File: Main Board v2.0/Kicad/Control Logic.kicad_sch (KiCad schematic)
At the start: 24 parts, among them J2 +3V3 Supply, J3 JTAG, U7 XC95288XL-TQ144, U8 AP1117-33

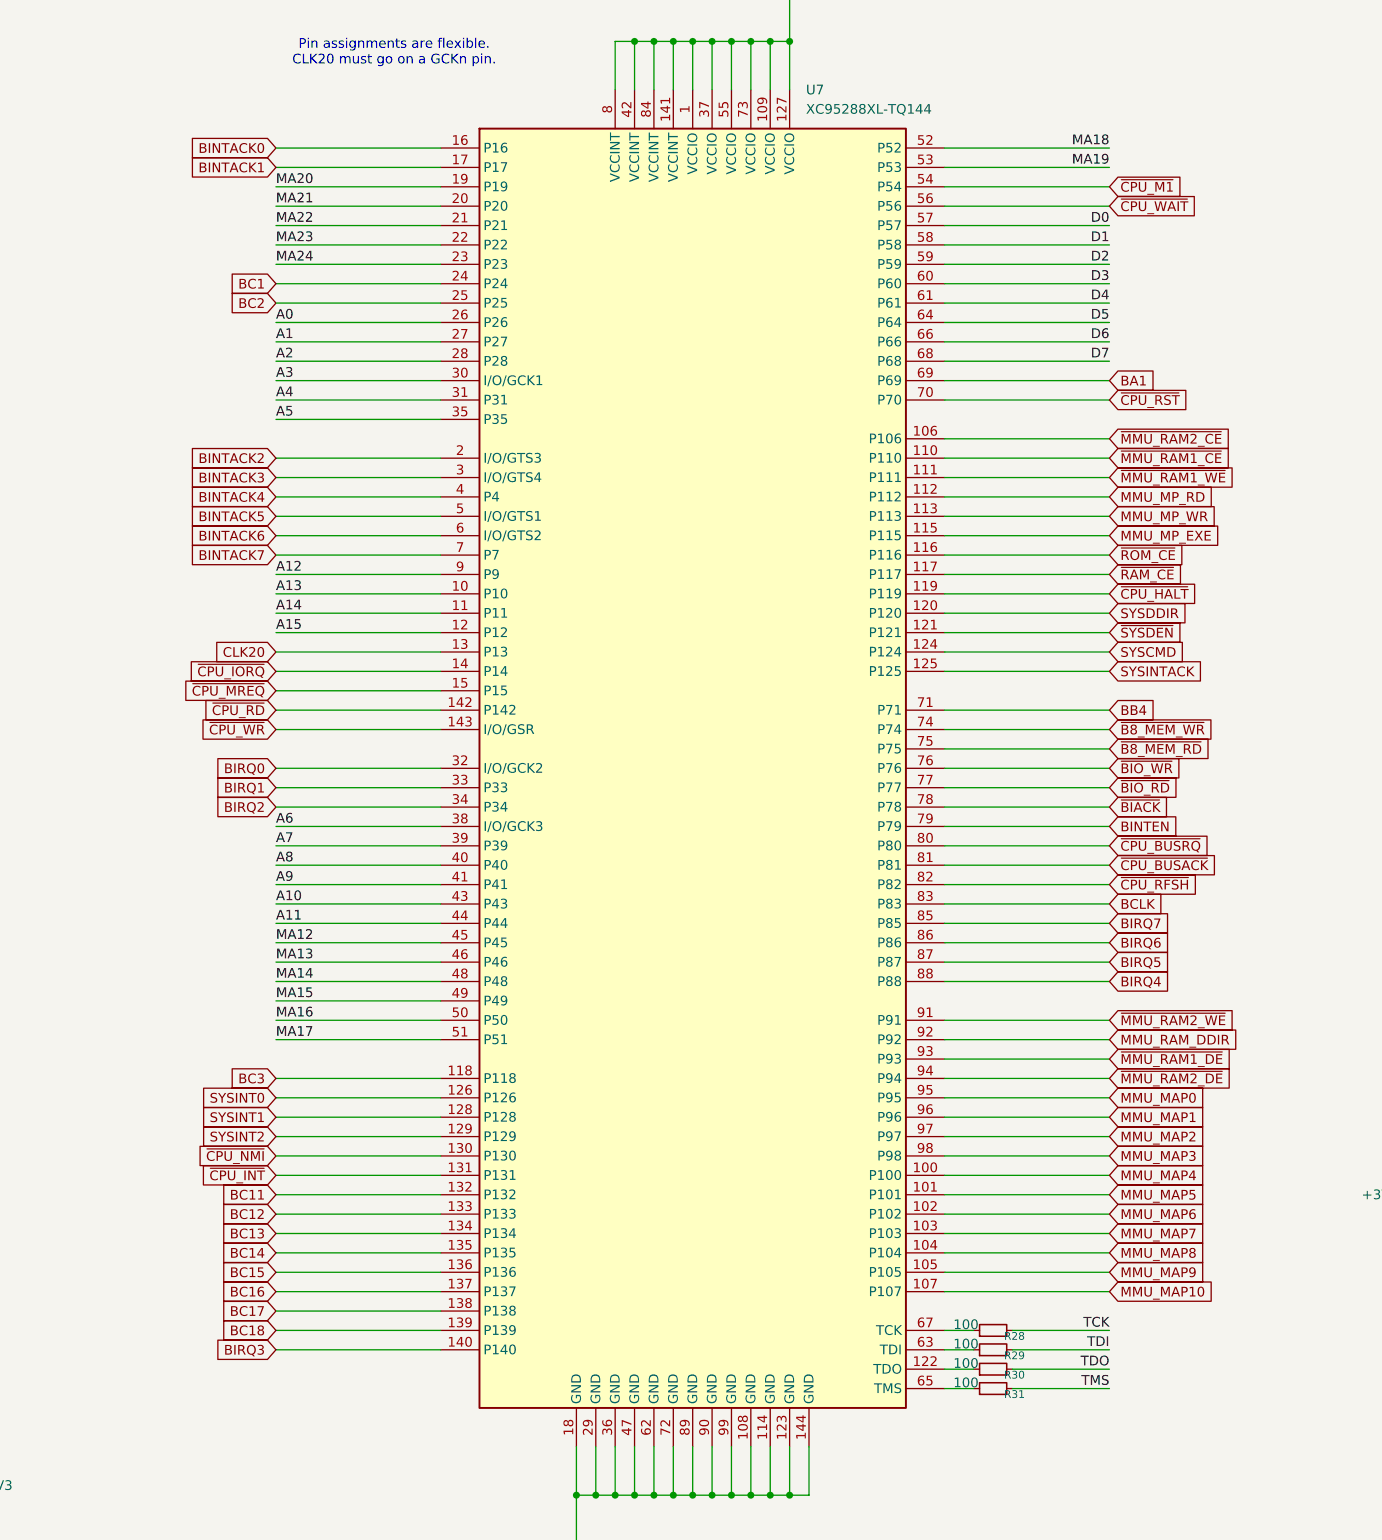
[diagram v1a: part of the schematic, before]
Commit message: board update
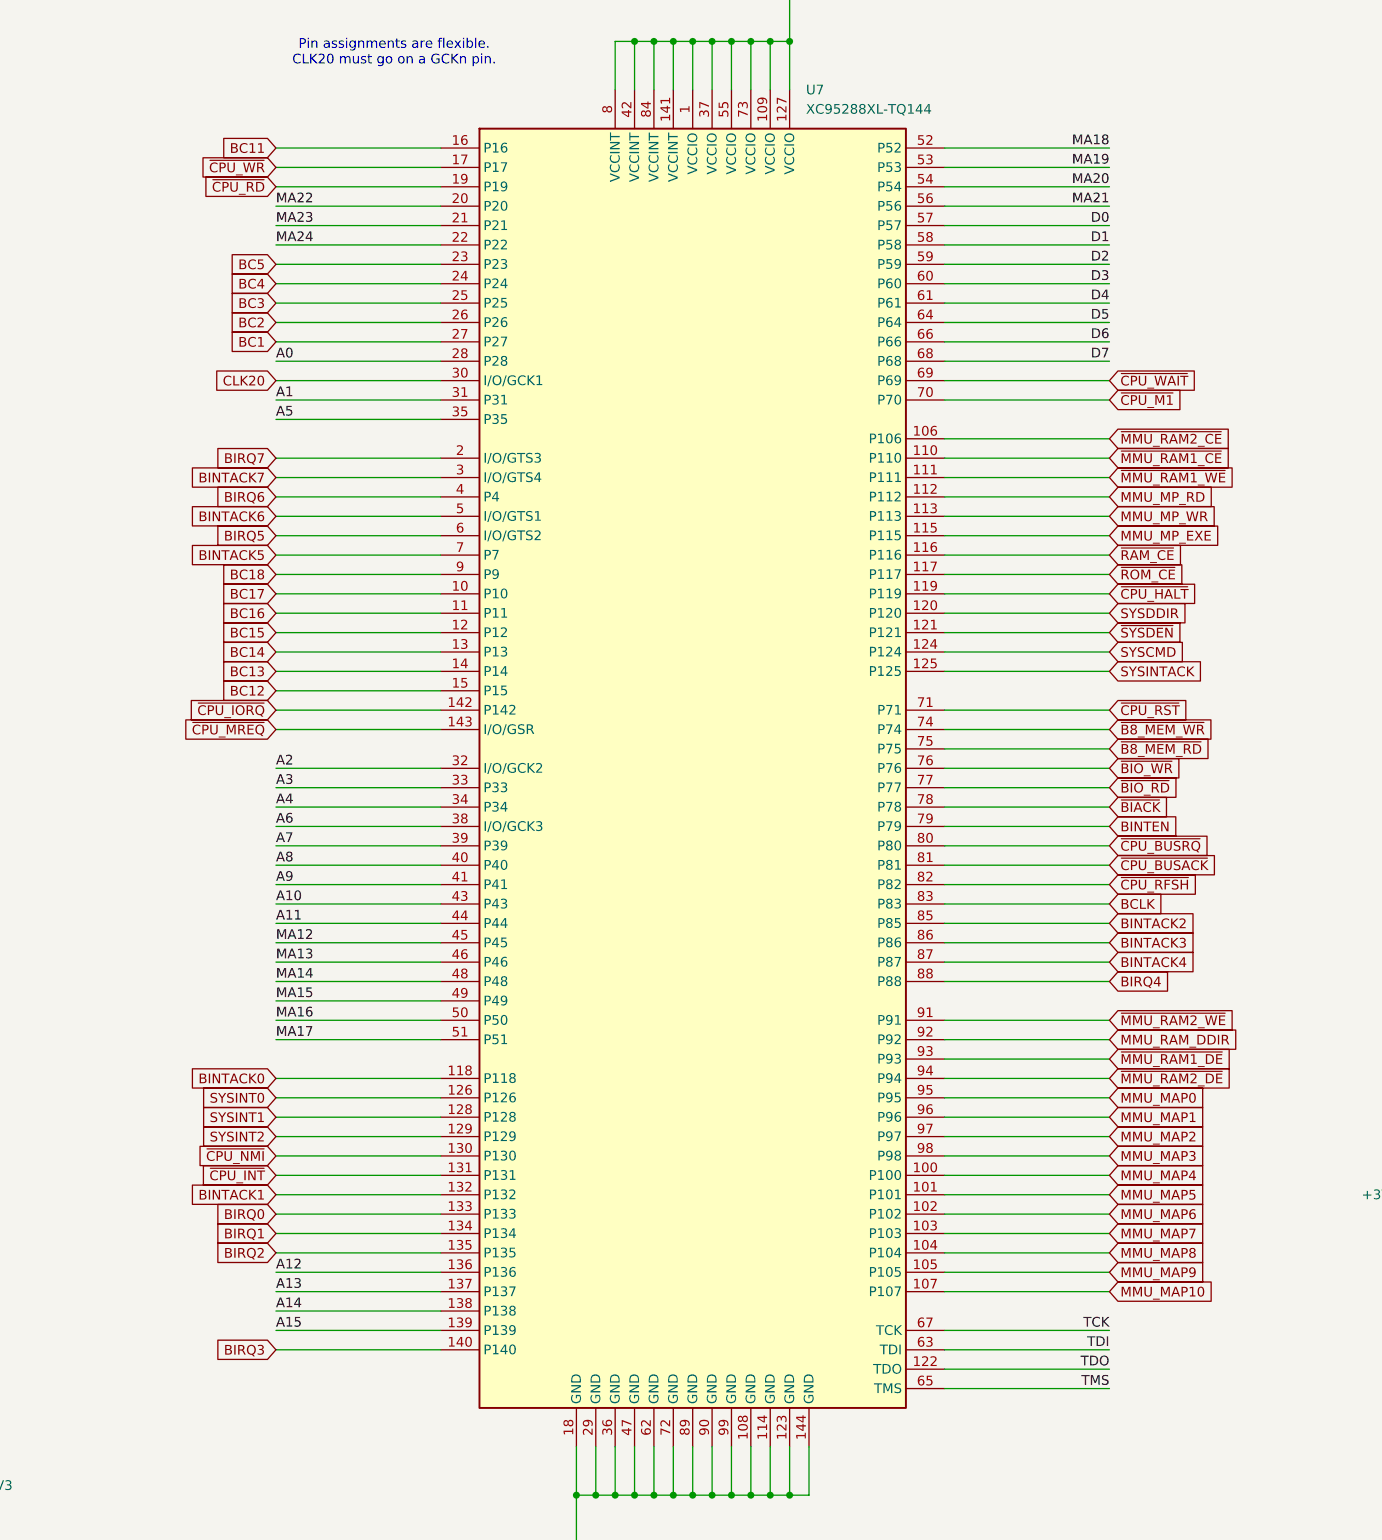
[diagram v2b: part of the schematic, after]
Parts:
- removed R28, R29, R30, R31: 100, Resistor_SMD:R_0603_1608Metric_Pad0.98x0.95mm_HandSolder, symbol Device:R_Small
- C10, C11, C12, C13, C14, C15, C16, C17, C7, C8, C9, R32, R33, R34: KiLib_Generator (none) -> SMD_2terminal_chip_molded
- C18, C19: KiLib_Generator (none) -> capacitor/THT/other
- J2, J3: KiLib_Generator (none) -> connector/pin_header_socket
- U7: KiLib_Generator (none) -> package/gullwing
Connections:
- net BA1 is gone; now on net ~{CPU_WAIT}: U7.69 (P69)
- net BB4 is gone; now on net ~{CPU_RST}: U7.71 (P71)
- net A0: now also U7.28 (P28); no longer U7.26 (P26)
- net A1: now also U7.31 (P31); no longer U7.27 (P27)
- net A12: now also U7.136 (P136); no longer U7.9 (P9)
- net A13: now also U7.137 (P137); no longer U7.10 (P10)
- net A14: now also U7.138 (P138); no longer U7.11 (P11)
- net A15: now also U7.139 (P139); no longer U7.12 (P12)
- net A2: now also U7.32 (I/O/GCK2); no longer U7.28 (P28)
- net A3: now also U7.33 (P33); no longer U7.30 (I/O/GCK1)
- net A4: now also U7.34 (P34); no longer U7.31 (P31)
- net BC1: now also U7.27 (P27); no longer U7.24 (P24)
- net BC11: now also U7.16 (P16); no longer U7.132 (P132)
- net BC12: now also U7.15 (P15); no longer U7.133 (P133)
- net BC13: now also U7.14 (P14); no longer U7.134 (P134)
- net BC14: now also U7.13 (P13); no longer U7.135 (P135)
- net BC15: now also U7.12 (P12); no longer U7.136 (P136)
- net BC16: now also U7.11 (P11); no longer U7.137 (P137)
- net BC17: now also U7.10 (P10); no longer U7.138 (P138)
- net BC18: now also U7.9 (P9); no longer U7.139 (P139)
- net BC2: now also U7.26 (P26); no longer U7.25 (P25)
- net BC3: now also U7.25 (P25); no longer U7.118 (P118)
- net BINTACK0: now also U7.118 (P118); no longer U7.16 (P16)
- net BINTACK1: now also U7.132 (P132); no longer U7.17 (P17)
- net BINTACK2: now also U7.85 (P85); no longer U7.2 (I/O/GTS3)
- net BINTACK3: now also U7.86 (P86); no longer U7.3 (I/O/GTS4)
- net BINTACK4: now also U7.87 (P87); no longer U7.4 (P4)
- net BINTACK5: now also U7.7 (P7); no longer U7.5 (I/O/GTS1)
- net BINTACK6: now also U7.5 (I/O/GTS1); no longer U7.6 (I/O/GTS2)
- net BINTACK7: now also U7.3 (I/O/GTS4); no longer U7.7 (P7)
- net BIRQ0: now also U7.133 (P133); no longer U7.32 (I/O/GCK2)
- net BIRQ1: now also U7.134 (P134); no longer U7.33 (P33)
- net BIRQ2: now also U7.135 (P135); no longer U7.34 (P34)
- net BIRQ5: now also U7.6 (I/O/GTS2); no longer U7.87 (P87)
- net BIRQ6: now also U7.4 (P4); no longer U7.86 (P86)
- net BIRQ7: now also U7.2 (I/O/GTS3); no longer U7.85 (P85)
- net CLK20: now also U7.30 (I/O/GCK1); no longer U7.13 (P13)
- net MA20: now also U7.54 (P54); no longer U7.19 (P19)
- net MA21: now also U7.56 (P56); no longer U7.20 (P20)
- net MA22: now also U7.20 (P20); no longer U7.21 (P21)
- net MA23: now also U7.21 (P21); no longer U7.22 (P22)
- net MA24: now also U7.22 (P22); no longer U7.23 (P23)
- net TCK: now also U7.67 (TCK)
- net TDI: now also U7.63 (TDI)
- net TDO: now also U7.122 (TDO)
- net TMS: now also U7.65 (TMS)
- net ~{CPU_IORQ}: now also U7.142 (P142); no longer U7.14 (P14)
- net ~{CPU_M1}: now also U7.70 (P70); no longer U7.54 (P54)
- net ~{CPU_MREQ}: now also U7.143 (I/O/GSR); no longer U7.15 (P15)
- net ~{CPU_RD}: now also U7.19 (P19); no longer U7.142 (P142)
- net ~{CPU_RST}: no longer U7.70 (P70)
- net ~{CPU_WAIT}: no longer U7.56 (P56)
- net ~{CPU_WR}: now also U7.17 (P17); no longer U7.143 (I/O/GSR)
- net ~{RAM_CE}: now also U7.116 (P116); no longer U7.117 (P117)
- net ~{ROM_CE}: now also U7.117 (P117); no longer U7.116 (P116)
- new net BC4: U7.24 (P24)
- new net BC5: U7.23 (P23)

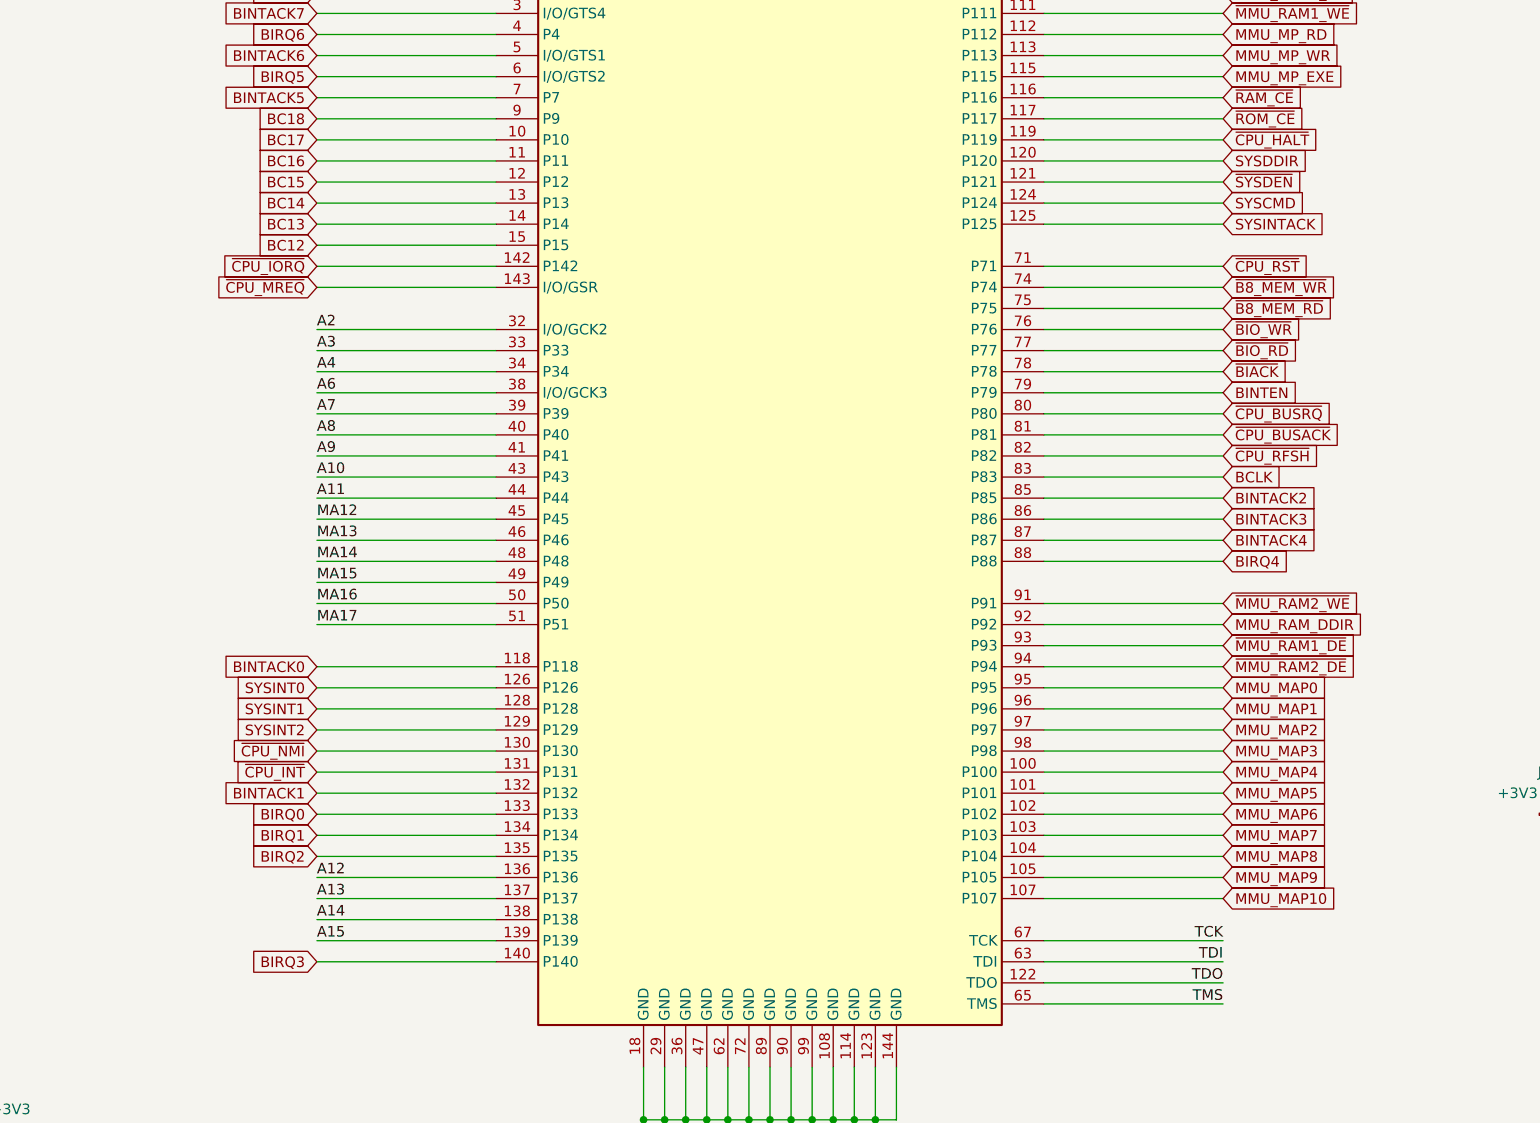
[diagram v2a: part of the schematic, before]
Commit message: board progress
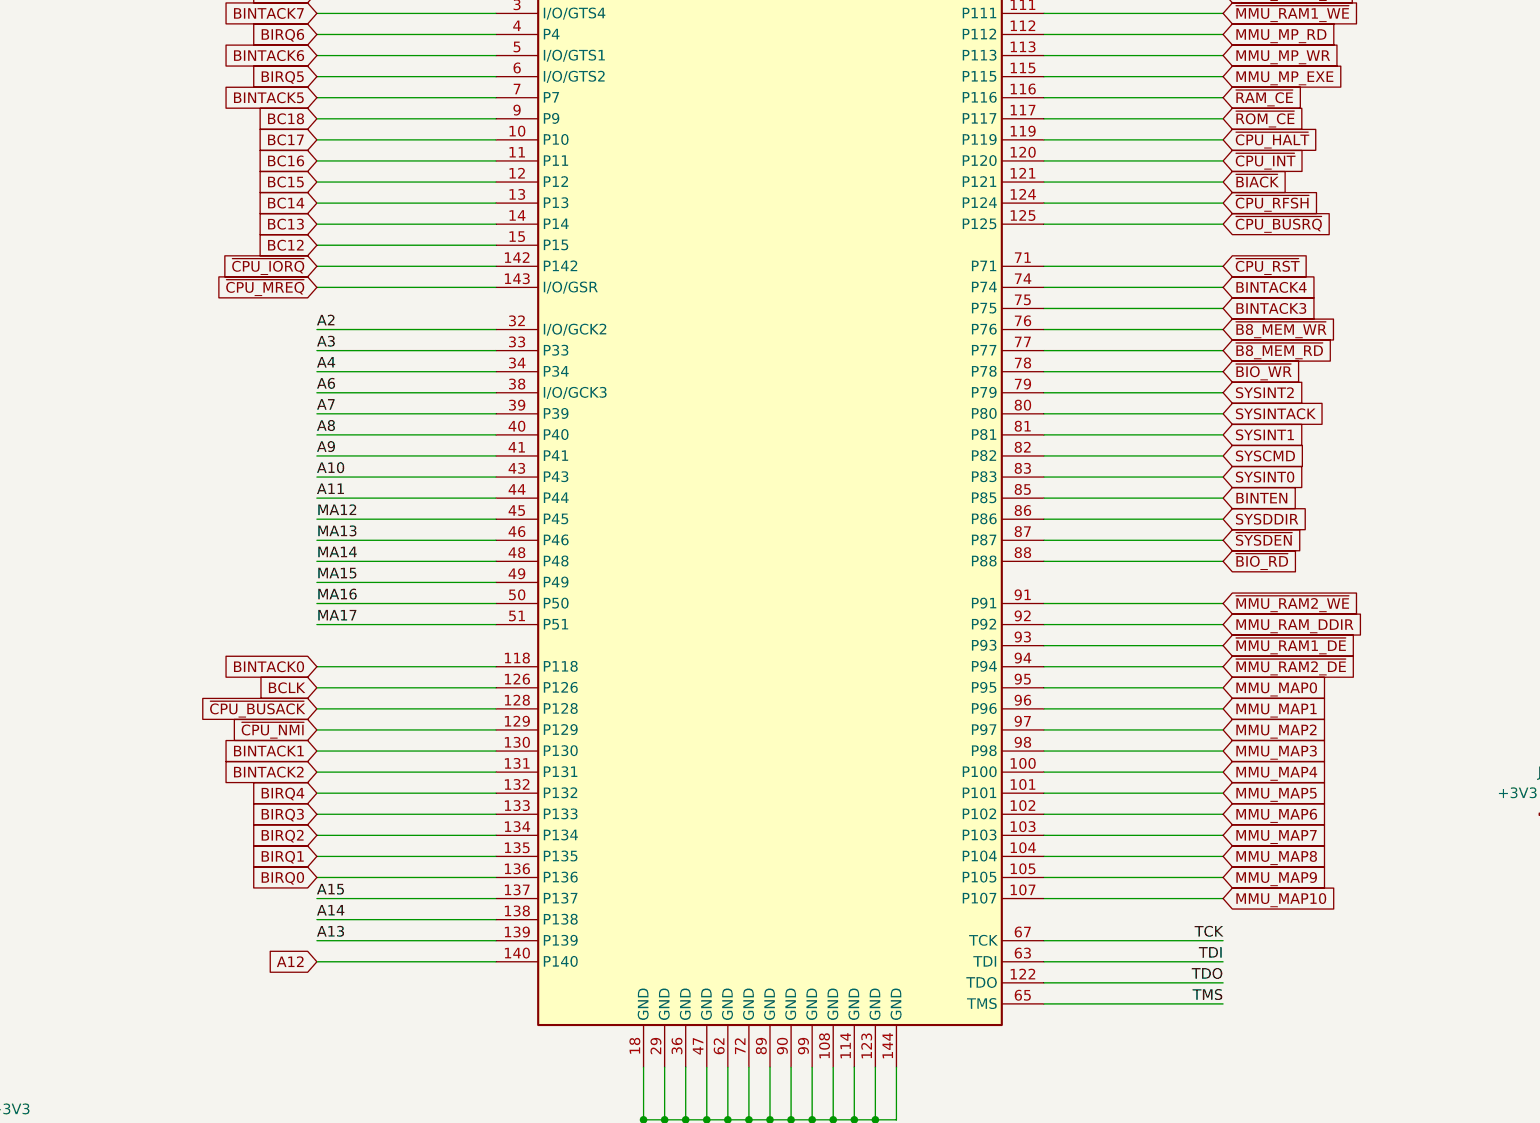
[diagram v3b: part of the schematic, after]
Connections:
- net A12: now also U7.140 (P140); no longer U7.136 (P136)
- net A13: now also U7.139 (P139); no longer U7.137 (P137)
- net A15: now also U7.137 (P137); no longer U7.139 (P139)
- net BCLK: now also U7.126 (P126); no longer U7.83 (P83)
- net BINTACK1: now also U7.130 (P130); no longer U7.132 (P132)
- net BINTACK2: now also U7.131 (P131); no longer U7.85 (P85)
- net BINTACK3: now also U7.75 (P75); no longer U7.86 (P86)
- net BINTACK4: now also U7.74 (P74); no longer U7.87 (P87)
- net BINTEN: now also U7.85 (P85); no longer U7.79 (P79)
- net BIRQ0: now also U7.136 (P136); no longer U7.133 (P133)
- net BIRQ1: now also U7.135 (P135); no longer U7.134 (P134)
- net BIRQ2: now also U7.134 (P134); no longer U7.135 (P135)
- net BIRQ3: now also U7.133 (P133); no longer U7.140 (P140)
- net BIRQ4: now also U7.132 (P132); no longer U7.88 (P88)
- net SYSCMD: now also U7.82 (P82); no longer U7.124 (P124)
- net SYSDDIR: now also U7.86 (P86); no longer U7.120 (P120)
- net SYSINT0: now also U7.83 (P83); no longer U7.126 (P126)
- net SYSINT1: now also U7.81 (P81); no longer U7.128 (P128)
- net SYSINT2: now also U7.79 (P79); no longer U7.129 (P129)
- net SYSINTACK: now also U7.80 (P80); no longer U7.125 (P125)
- net ~{B8_MEM_RD}: now also U7.77 (P77); no longer U7.75 (P75)
- net ~{B8_MEM_WR}: now also U7.76 (P76); no longer U7.74 (P74)
- net ~{BIACK}: now also U7.121 (P121); no longer U7.78 (P78)
- net ~{BIO_RD}: now also U7.88 (P88); no longer U7.77 (P77)
- net ~{BIO_WR}: now also U7.78 (P78); no longer U7.76 (P76)
- net ~{CPU_BUSACK}: now also U7.128 (P128); no longer U7.81 (P81)
- net ~{CPU_BUSRQ}: now also U7.125 (P125); no longer U7.80 (P80)
- net ~{CPU_INT}: now also U7.120 (P120); no longer U7.131 (P131)
- net ~{CPU_NMI}: now also U7.129 (P129); no longer U7.130 (P130)
- net ~{CPU_RFSH}: now also U7.124 (P124); no longer U7.82 (P82)
- net ~{SYSDEN}: now also U7.87 (P87); no longer U7.121 (P121)
